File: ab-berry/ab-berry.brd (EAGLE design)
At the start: 66 x 62.2 mm, 34 parts, among them U1 LM1117MPX-3.3/NOPB or AP2114H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

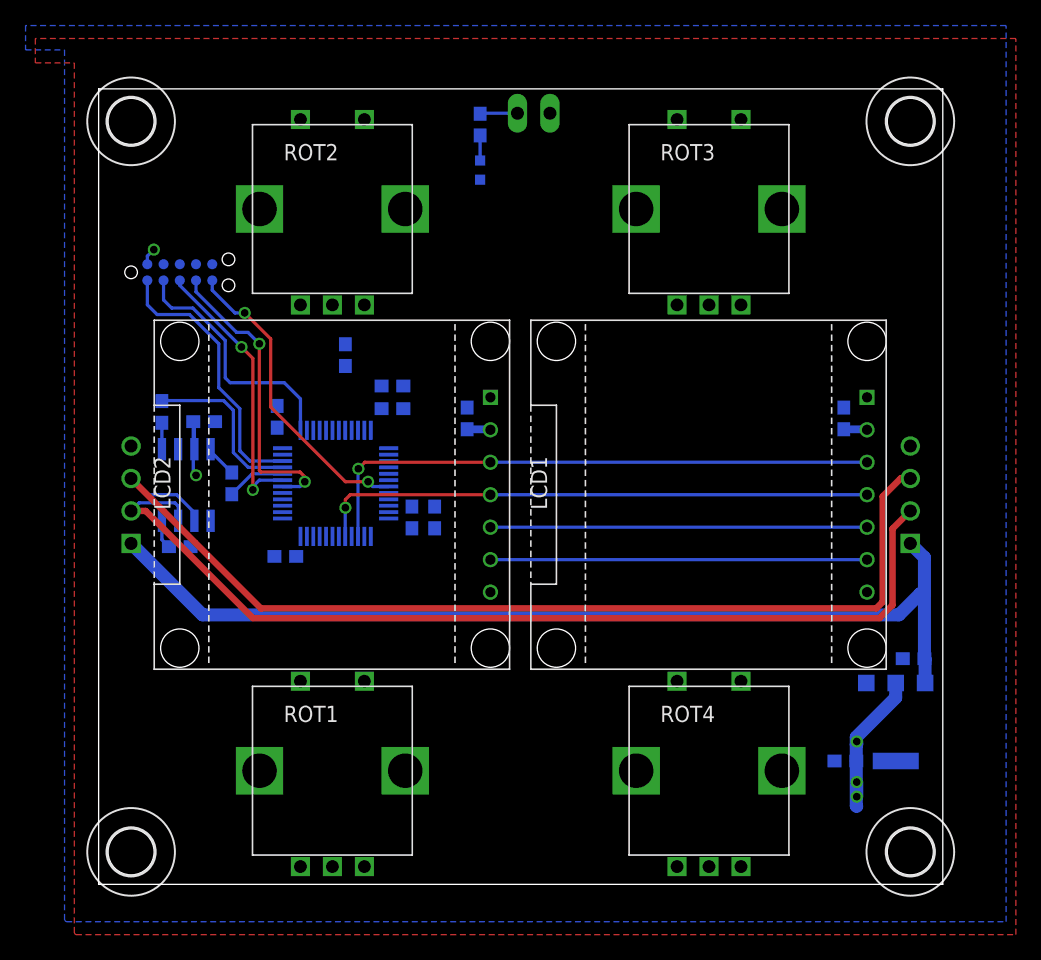
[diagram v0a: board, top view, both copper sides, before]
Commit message: wip
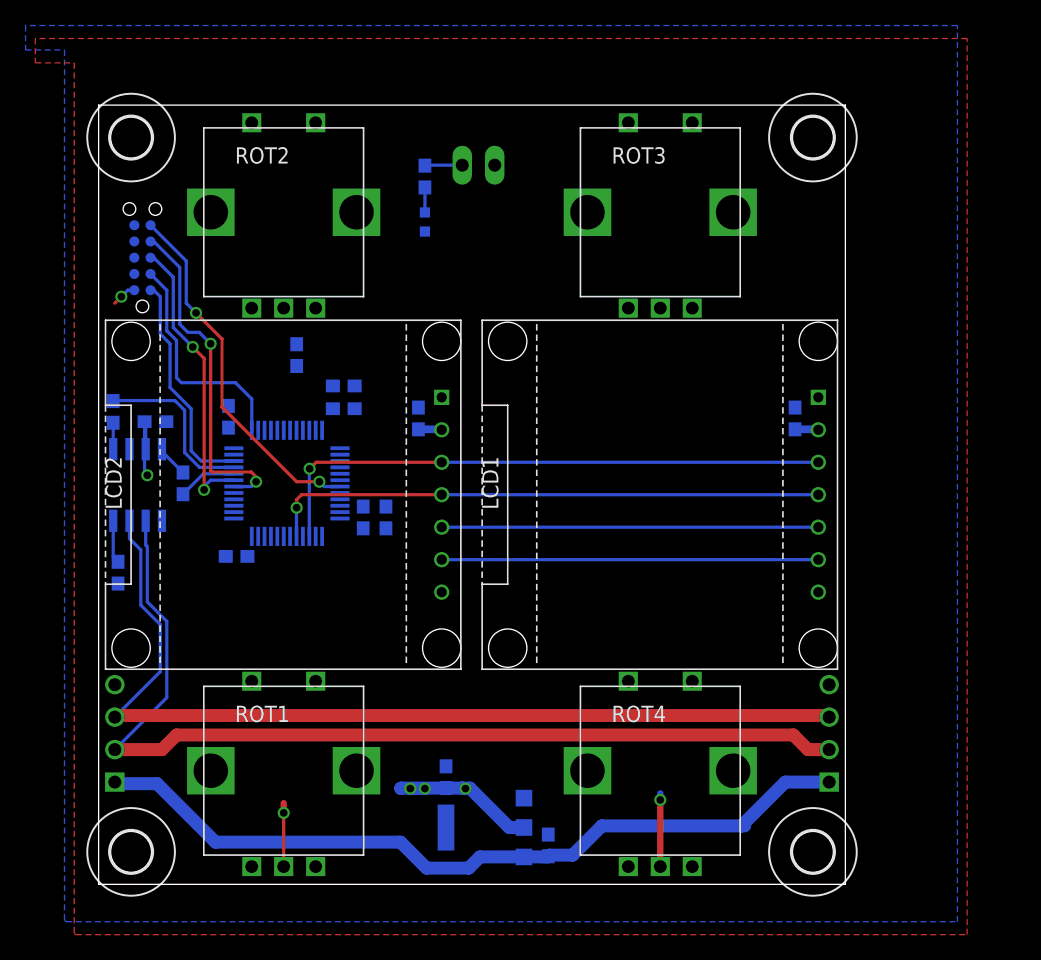
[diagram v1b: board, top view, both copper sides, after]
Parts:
- H1, H2, H3, H4: value MOUNT-HOLE3.6 -> MOUNT-HOLE3.2; device holes:3,6 -> holes:3,2
- moved U1 33.2 mm to (30.2, 4.45), turned to 270 degrees
- moved C8 32.1 mm to (35.2, 3.05), turned to 270 degrees
- moved C9 31.3 mm to (27.2, 8.38), turned to 90 degrees
- moved JP2 19.7 mm to (57.1, 11.8)
- moved JP1 18.7 mm to (1.27, 11.8)
- moved H3 7.73 mm to (55.9, 58.4)
- moved H4 7.62 mm to (55.9, 2.54)
- moved JP3 5.93 mm to (29.7, 56.3)
- moved LED1 5.93 mm to (25.5, 51.8)
- moved R5 5.93 mm to (25.5, 55.4)
- moved R2 5.24 mm to (1.52, 24.4), turned to 270 degrees
- moved ROT3 3.82 mm to (43.9, 52.6)
- moved ROT2 3.82 mm to (14.5, 52.6)
- moved C10 3.81 mm to (54.5, 36.4)
- moved C11 3.81 mm to (25.0, 36.4)
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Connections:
- net CAN_H: now also JP1.3, JP2.3; no longer JP1.2, JP2.2
- net CAN_L: now also JP1.2, JP2.2; no longer JP1.3, JP2.3
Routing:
- net 5.0V: track 76.5 -> 61.7 mm
- net GND: track 0.00 -> 10.7 mm, vias 0 -> 2
- net RST: track 24.1 -> 28.3 mm
- net CAN_L: track 80.9 -> 77.1 mm
- net SWDIO: track 21.5 -> 17.7 mm
- net DBG_TX: track 23.5 -> 26.6 mm
- net CAN_H: track 76.6 -> 73.8 mm
- net SWCLK: track 19.6 -> 18.0 mm
- net DBG_RX: track 21.5 -> 22.8 mm
- net N$2: track 2.25 -> 3.37 mm
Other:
- board size 66 x 62.2 mm -> 58.4 x 61 mm
